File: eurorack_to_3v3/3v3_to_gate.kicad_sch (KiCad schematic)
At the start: 17 parts, among them U1 LM324

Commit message: fix gate_to_3v3 schematic
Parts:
- U1: symbol Device:Opamp_Quad_Generic -> Device:Opamp_Quad
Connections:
- net +12V: now also U1.4 (V+)
- net -12V: now also U1.11 (V-)
- net at R5.1, R7.2: now also U1.1
- net at R3.1, R5.2: now also U1.2 (-)
- net at R1.1: now also U1.3 (+)
- net at R6.1, R8.2: now also U1.8
- net at R4.1, R6.2: now also U1.9 (-)
- net at R2.1: now also U1.10 (+)
- net at R13.1, R15.2: now also U1.7
- net at R11.1, R13.2: now also U1.6 (-)
- net at R9.1: now also U1.5 (+)
- net at R14.1, R16.2: now also U1.14
- net at R12.1, R14.2: now also U1.13 (-)
- net at R10.1: now also U1.12 (+)
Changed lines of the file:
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@@
     (effects (font (size 1.27 1.27) italic) (justify right))
   )
-  (symbol (lib_id "Device:Opamp_Quad_Generic") (at 100.711 65.913 0) (unit 1)
+  (symbol (lib_id "Device:Opamp_Quad") (at 100.711 65.913 0) (unit 1)
     (in_bom yes) (on_board yes)
     (property "Reference" "U1" (id 0) (at 100.711 56.5912 0))
@@
       (effects (font (size 1.27 1.27)) hide)
     )
+    (pin "1")
+    (pin "2")
+    (pin "3")
   )
   (symbol (lib_id "Device:R_US") (at 115.951 65.913 270) (unit 1)
@@
     (pin "1")
   )
-  (symbol (lib_id "Device:Opamp_Quad_Generic") (at 100.711 120.523 0) (unit 3)
+  (symbol (lib_id "Device:Opamp_Quad") (at 100.711 120.523 0) (unit 3)
     (in_bom yes) (on_board yes)
     (property "Reference" "U1" (id 0) (at 100.711 111.2012 0))
@@
       (effects (font (size 1.27 1.27)) hide)
     )
+    (pin "10")
+    (pin "8")
+    (pin "9")
   )
   (symbol (lib_id "Device:R_US") (at 115.951 120.523 270) (unit 1)
@@
     (pin "1")
   )
-  (symbol (lib_id "Device:Opamp_Quad_Generic") (at 200.025 65.913 0) (unit 2)
+  (symbol (lib_id "Device:Opamp_Quad") (at 200.025 65.913 0) (unit 2)
     (in_bom yes) (on_board yes)
     (property "Reference" "U1" (id 0) (at 200.025 56.5912 0))
@@
       (effects (font (size 1.27 1.27)) hide)
     )
+    (pin "5")
+    (pin "6")
+    (pin "7")
   )
   (symbol (lib_id "Device:R_US") (at 215.265 65.913 270) (unit 1)
@@
     (pin "1")
   )
-  (symbol (lib_id "Device:Opamp_Quad_Generic") (at 200.025 120.523 0) (unit 4)
+  (symbol (lib_id "Device:Opamp_Quad") (at 200.025 120.523 0) (unit 4)
     (in_bom yes) (on_board yes)
     (property "Reference" "U1" (id 0) (at 200.025 111.2012 0))
@@
       (effects (font (size 1.27 1.27)) hide)
     )
+    (pin "12")
+    (pin "13")
+    (pin "14")
   )
   (symbol (lib_id "Device:R_US") (at 215.265 120.523 270) (unit 1)
@@
     (pin "1")
   )
-  (symbol (lib_id "Device:Opamp_Quad_Generic") (at 148.59 93.345 0) (unit 5)
+  (symbol (lib_id "Device:Opamp_Quad") (at 148.59 93.345 0) (unit 5)
     (in_bom yes) (on_board yes)
     (property "Reference" "U1" (id 0) (at 149.86 91.44 0))
@@
       (effects (font (size 1.27 1.27)) hide)
     )
+    (pin "11")
+    (pin "4")
   )
   (symbol (lib_id "power:+12V") (at 146.05 85.725 0) (unit 1)

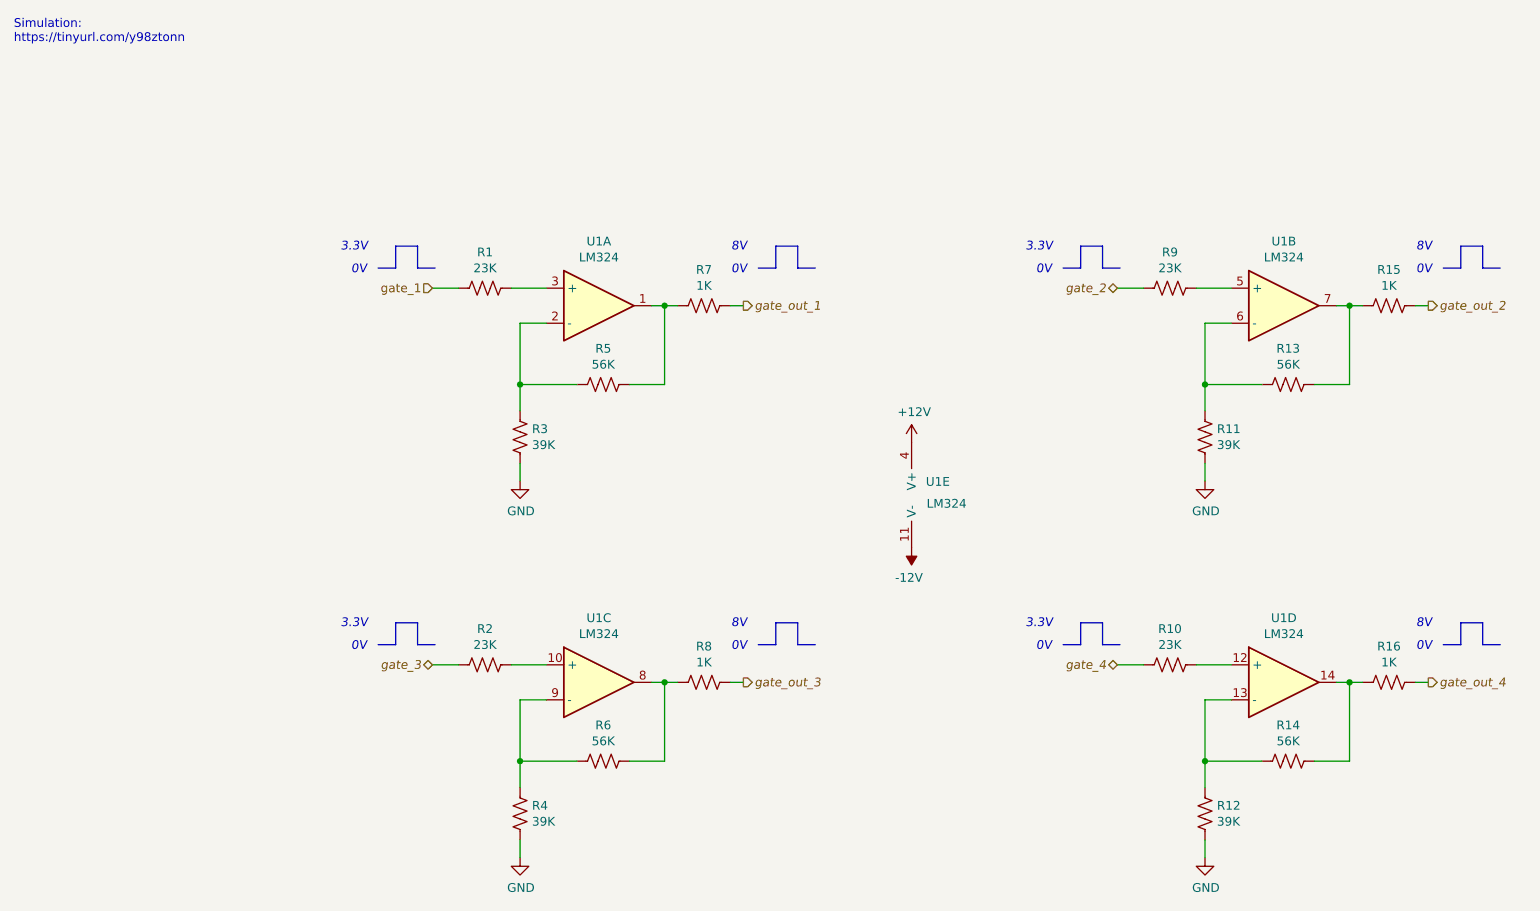
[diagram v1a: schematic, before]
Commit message: finished Big One Little One v2
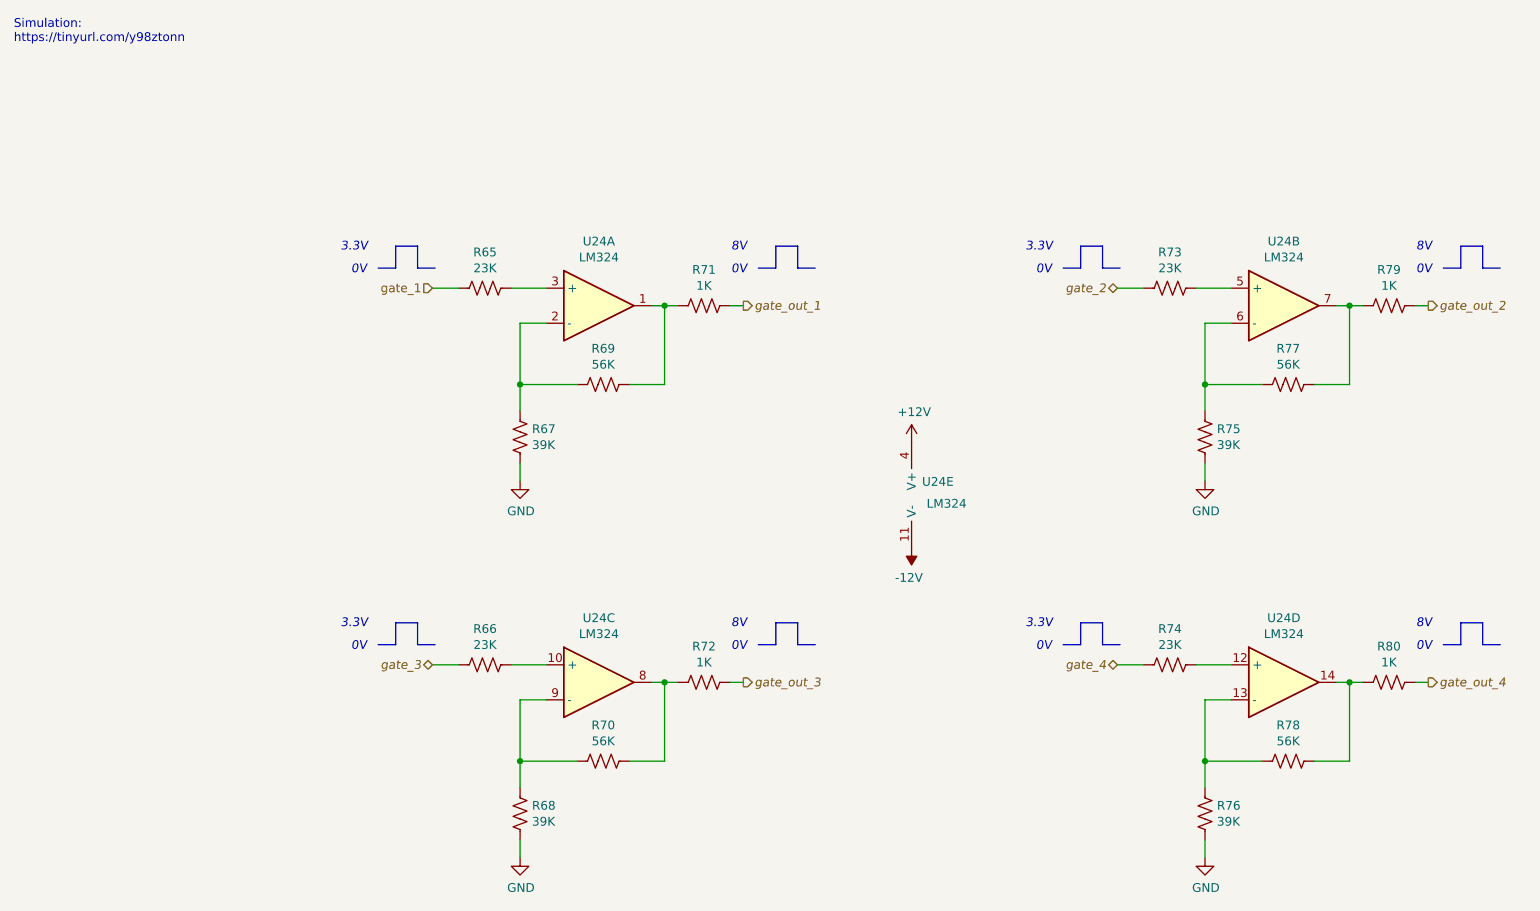
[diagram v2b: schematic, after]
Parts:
- renumbered R1 to R65, R2 to R66, R3 to R67, R4 to R68, R5 to R69, R6 to R70, R7 to R71, R8 to R72, R9 to R73, R10 to R74, R11 to R75, R12 to R76, R13 to R77, R14 to R78, R15 to R79, R16 to R80, U1 to U24
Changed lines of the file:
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@@
   (symbol (lib_id "Device:Opamp_Quad") (at 100.711 65.913 0) (unit 1)
     (in_bom yes) (on_board yes)
-    (property "Reference" "U1" (id 0) (at 100.711 56.5912 0))
+    (property "Reference" "U24" (id 0) (at 100.711 56.5912 0))
     (property "Value" "LM324" (id 1) (at 100.711 58.9026 0))
     (property "Footprint" "Package_SO:SOIC-14_3.9x8.7mm_P1.27mm" (id 2) (at 100.711 65.913 0)
@@
   (symbol (lib_id "Device:R_US") (at 115.951 65.913 270) (unit 1)
     (in_bom yes) (on_board yes)
-    (property "Reference" "R7" (id 0) (at 115.951 60.706 90))
+    (property "Reference" "R71" (id 0) (at 115.951 60.706 90))
     (property "Value" "1K" (id 1) (at 115.951 63.0174 90))
     (property "Footprint" "Resistor_SMD:R_0402_1005Metric" (id 2) (at 115.697 66.929 90)
@@
   (symbol (lib_id "Device:R_US") (at 101.346 77.343 270) (unit 1)
     (in_bom yes) (on_board yes)
-    (property "Reference" "R5" (id 0) (at 101.346 72.136 90))
+    (property "Reference" "R69" (id 0) (at 101.346 72.136 90))
     (property "Value" "56K" (id 1) (at 101.346 74.4474 90))
     (property "Footprint" "Resistor_SMD:R_0402_1005Metric" (id 2) (at 101.092 78.359 90)
@@
   (symbol (lib_id "Device:R_US") (at 89.281 84.963 0) (unit 1)
     (in_bom yes) (on_board yes)
-    (property "Reference" "R3" (id 0) (at 91.0082 83.7946 0)
+    (property "Reference" "R67" (id 0) (at 91.0082 83.7946 0)
       (effects (font (size 1.27 1.27)) (justify left))
     )
@@
   (symbol (lib_id "Device:R_US") (at 84.201 63.373 270) (unit 1)
     (in_bom yes) (on_board yes)
-    (property "Reference" "R1" (id 0) (at 84.201 58.166 90))
+    (property "Reference" "R65" (id 0) (at 84.201 58.166 90))
     (property "Value" "23K" (id 1) (at 84.201 60.4774 90))
     (property "Footprint" "Resistor_SMD:R_0402_1005Metric" (id 2) (at 83.947 64.389 90)
@@
   (symbol (lib_id "power:GND") (at 89.281 91.313 0) (unit 1)
     (in_bom yes) (on_board yes)
-    (property "Reference" "#PWR01" (id 0) (at 89.281 97.663 0)
+    (property "Reference" "#PWR092" (id 0) (at 89.281 97.663 0)
       (effects (font (size 1.27 1.27)) hide)
     )
@@
   (symbol (lib_id "Device:Opamp_Quad") (at 100.711 120.523 0) (unit 3)
     (in_bom yes) (on_board yes)
-    (property "Reference" "U1" (id 0) (at 100.711 111.2012 0))
+    (property "Reference" "U24" (id 0) (at 100.711 111.2012 0))
     (property "Value" "LM324" (id 1) (at 100.711 113.5126 0))
     (property "Footprint" "Package_SO:SOIC-14_3.9x8.7mm_P1.27mm" (id 2) (at 100.711 120.523 0)
@@
   (symbol (lib_id "Device:R_US") (at 115.951 120.523 270) (unit 1)
     (in_bom yes) (on_board yes)
-    (property "Reference" "R8" (id 0) (at 115.951 115.316 90))
+    (property "Reference" "R72" (id 0) (at 115.951 115.316 90))
     (property "Value" "1K" (id 1) (at 115.951 117.6274 90))
     (property "Footprint" "Resistor_SMD:R_0402_1005Metric" (id 2) (at 115.697 121.539 90)
@@
   (symbol (lib_id "Device:R_US") (at 101.346 131.953 270) (unit 1)
     (in_bom yes) (on_board yes)
-    (property "Reference" "R6" (id 0) (at 101.346 126.746 90))
+    (property "Reference" "R70" (id 0) (at 101.346 126.746 90))
     (property "Value" "56K" (id 1) (at 101.346 129.0574 90))
     (property "Footprint" "Resistor_SMD:R_0402_1005Metric" (id 2) (at 101.092 132.969 90)
@@
   (symbol (lib_id "Device:R_US") (at 89.281 139.573 0) (unit 1)
     (in_bom yes) (on_board yes)
-    (property "Reference" "R4" (id 0) (at 91.0082 138.4046 0)
+    (property "Reference" "R68" (id 0) (at 91.0082 138.4046 0)
       (effects (font (size 1.27 1.27)) (justify left))
     )
@@
   (symbol (lib_id "Device:R_US") (at 84.201 117.983 270) (unit 1)
     (in_bom yes) (on_board yes)
-    (property "Reference" "R2" (id 0) (at 84.201 112.776 90))
+    (property "Reference" "R66" (id 0) (at 84.201 112.776 90))
     (property "Value" "23K" (id 1) (at 84.201 115.0874 90))
     (property "Footprint" "Resistor_SMD:R_0402_1005Metric" (id 2) (at 83.947 118.999 90)
@@
   (symbol (lib_id "power:GND") (at 89.281 145.923 0) (unit 1)
     (in_bom yes) (on_board yes)
-    (property "Reference" "#PWR02" (id 0) (at 89.281 152.273 0)
+    (property "Reference" "#PWR093" (id 0) (at 89.281 152.273 0)
       (effects (font (size 1.27 1.27)) hide)
     )
@@
   (symbol (lib_id "Device:Opamp_Quad") (at 200.025 65.913 0) (unit 2)
     (in_bom yes) (on_board yes)
-    (property "Reference" "U1" (id 0) (at 200.025 56.5912 0))
+    (property "Reference" "U24" (id 0) (at 200.025 56.5912 0))
     (property "Value" "LM324" (id 1) (at 200.025 58.9026 0))
     (property "Footprint" "Package_SO:SOIC-14_3.9x8.7mm_P1.27mm" (id 2) (at 200.025 65.913 0)
@@
   (symbol (lib_id "Device:R_US") (at 215.265 65.913 270) (unit 1)
     (in_bom yes) (on_board yes)
-    (property "Reference" "R15" (id 0) (at 215.265 60.706 90))
+    (property "Reference" "R79" (id 0) (at 215.265 60.706 90))
     (property "Value" "1K" (id 1) (at 215.265 63.0174 90))
     (property "Footprint" "Resistor_SMD:R_0402_1005Metric" (id 2) (at 215.011 66.929 90)
@@
   (symbol (lib_id "Device:R_US") (at 200.66 77.343 270) (unit 1)
     (in_bom yes) (on_board yes)
-    (property "Reference" "R13" (id 0) (at 200.66 72.136 90))
+    (property "Reference" "R77" (id 0) (at 200.66 72.136 90))
     (property "Value" "56K" (id 1) (at 200.66 74.4474 90))
     (property "Footprint" "Resistor_SMD:R_0402_1005Metric" (id 2) (at 200.406 78.359 90)
@@
   (symbol (lib_id "Device:R_US") (at 188.595 84.963 0) (unit 1)
     (in_bom yes) (on_board yes)
-    (property "Reference" "R11" (id 0) (at 190.3222 83.7946 0)
+    (property "Reference" "R75" (id 0) (at 190.3222 83.7946 0)
       (effects (font (size 1.27 1.27)) (justify left))
     )
@@
   (symbol (lib_id "Device:R_US") (at 183.515 63.373 270) (unit 1)
     (in_bom yes) (on_board yes)
-    (property "Reference" "R9" (id 0) (at 183.515 58.166 90))
+    (property "Reference" "R73" (id 0) (at 183.515 58.166 90))
     (property "Value" "23K" (id 1) (at 183.515 60.4774 90))
     (property "Footprint" "Resistor_SMD:R_0402_1005Metric" (id 2) (at 183.261 64.389 90)
@@
   (symbol (lib_id "power:GND") (at 188.595 91.313 0) (unit 1)
     (in_bom yes) (on_board yes)
-    (property "Reference" "#PWR03" (id 0) (at 188.595 97.663 0)
+    (property "Reference" "#PWR096" (id 0) (at 188.595 97.663 0)
       (effects (font (size 1.27 1.27)) hide)
     )
@@
   (symbol (lib_id "Device:Opamp_Quad") (at 200.025 120.523 0) (unit 4)
     (in_bom yes) (on_board yes)
-    (property "Reference" "U1" (id 0) (at 200.025 111.2012 0))
+    (property "Reference" "U24" (id 0) (at 200.025 111.2012 0))
     (property "Value" "LM324" (id 1) (at 200.025 113.5126 0))
     (property "Footprint" "Package_SO:SOIC-14_3.9x8.7mm_P1.27mm" (id 2) (at 200.025 120.523 0)
@@
   (symbol (lib_id "Device:R_US") (at 215.265 120.523 270) (unit 1)
     (in_bom yes) (on_board yes)
-    (property "Reference" "R16" (id 0) (at 215.265 115.316 90))
+    (property "Reference" "R80" (id 0) (at 215.265 115.316 90))
     (property "Value" "1K" (id 1) (at 215.265 117.6274 90))
     (property "Footprint" "Resistor_SMD:R_0402_1005Metric" (id 2) (at 215.011 121.539 90)
@@
   (symbol (lib_id "Device:R_US") (at 200.66 131.953 270) (unit 1)
     (in_bom yes) (on_board yes)
-    (property "Reference" "R14" (id 0) (at 200.66 126.746 90))
+    (property "Reference" "R78" (id 0) (at 200.66 126.746 90))
     (property "Value" "56K" (id 1) (at 200.66 129.0574 90))
     (property "Footprint" "Resistor_SMD:R_0402_1005Metric" (id 2) (at 200.406 132.969 90)
@@
   (symbol (lib_id "Device:R_US") (at 188.595 139.573 0) (unit 1)
     (in_bom yes) (on_board yes)
-    (property "Reference" "R12" (id 0) (at 190.3222 138.4046 0)
+    (property "Reference" "R76" (id 0) (at 190.3222 138.4046 0)
       (effects (font (size 1.27 1.27)) (justify left))
     )
@@
   (symbol (lib_id "Device:R_US") (at 183.515 117.983 270) (unit 1)
     (in_bom yes) (on_board yes)
-    (property "Reference" "R10" (id 0) (at 183.515 112.776 90))
+    (property "Reference" "R74" (id 0) (at 183.515 112.776 90))
     (property "Value" "23K" (id 1) (at 183.515 115.0874 90))
     (property "Footprint" "Resistor_SMD:R_0402_1005Metric" (id 2) (at 183.261 118.999 90)
@@
   (symbol (lib_id "power:GND") (at 188.595 145.923 0) (unit 1)
     (in_bom yes) (on_board yes)
-    (property "Reference" "#PWR04" (id 0) (at 188.595 152.273 0)
+    (property "Reference" "#PWR097" (id 0) (at 188.595 152.273 0)
       (effects (font (size 1.27 1.27)) hide)
     )
@@
   (symbol (lib_id "Device:Opamp_Quad") (at 148.59 93.345 0) (unit 5)
     (in_bom yes) (on_board yes)
-    (property "Reference" "U1" (id 0) (at 149.86 91.44 0))
+    (property "Reference" "U24" (id 0) (at 149.86 91.44 0))
     (property "Value" "LM324" (id 1) (at 151.13 94.615 0))
     (property "Footprint" "Package_SO:SOIC-14_3.9x8.7mm_P1.27mm" (id 2) (at 148.59 93.345 0)
@@
   (symbol (lib_id "power:+12V") (at 146.05 85.725 0) (unit 1)
     (in_bom yes) (on_board yes)
-    (property "Reference" "#PWR090" (id 0) (at 146.05 89.535 0)
+    (property "Reference" "#PWR094" (id 0) (at 146.05 89.535 0)
       (effects (font (size 1.27 1.27)) hide)
     )
@@
   (symbol (lib_id "power:-12V") (at 146.05 100.965 180) (unit 1)
     (in_bom yes) (on_board yes)
-    (property "Reference" "#PWR091" (id 0) (at 146.05 103.505 0)
-      (effects (font (size 1.27 1.27)) hide)
-    )
+    (property "Reference" "#PWR095" (id 0) (at 146.05 103.505 0)
+      (effects (font (size 1.27 1.27)) hide)
+    )
